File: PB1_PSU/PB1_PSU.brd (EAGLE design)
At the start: 100 x 80 mm, 0 parts

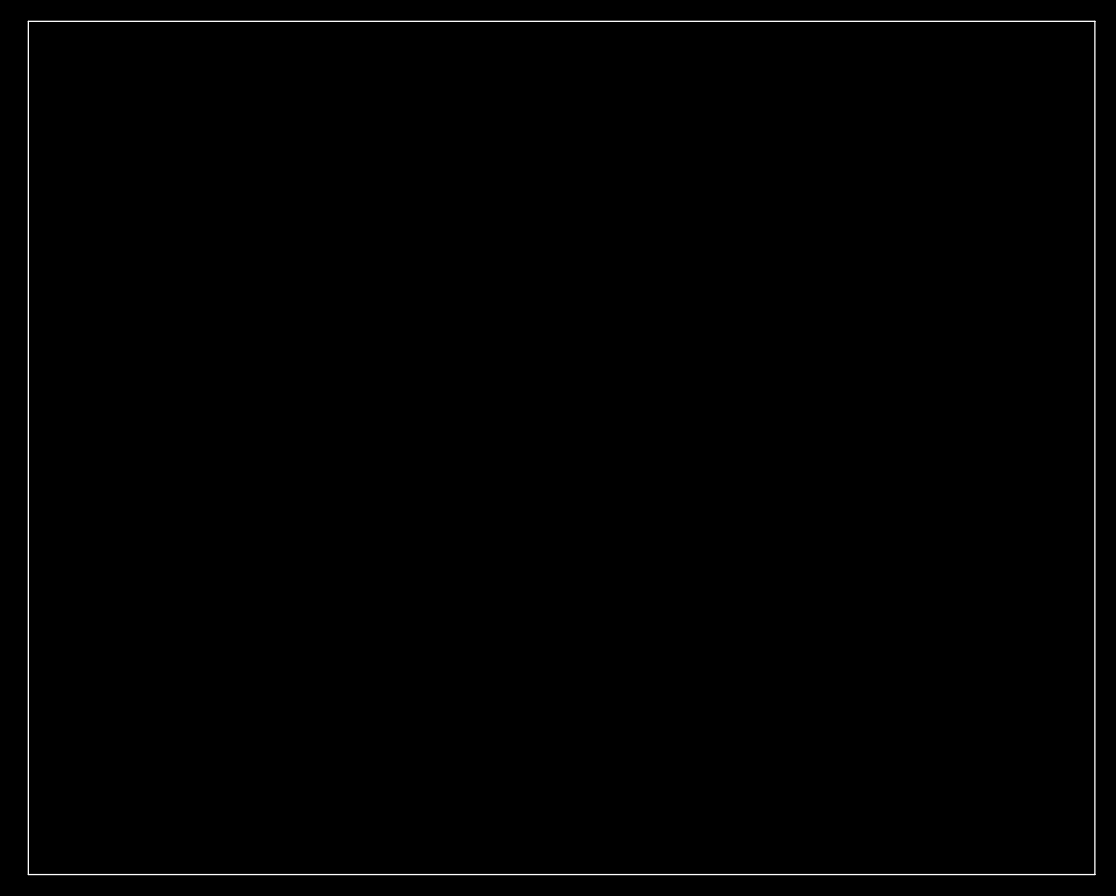
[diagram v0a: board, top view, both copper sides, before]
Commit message: * started on the PB1 powersupply
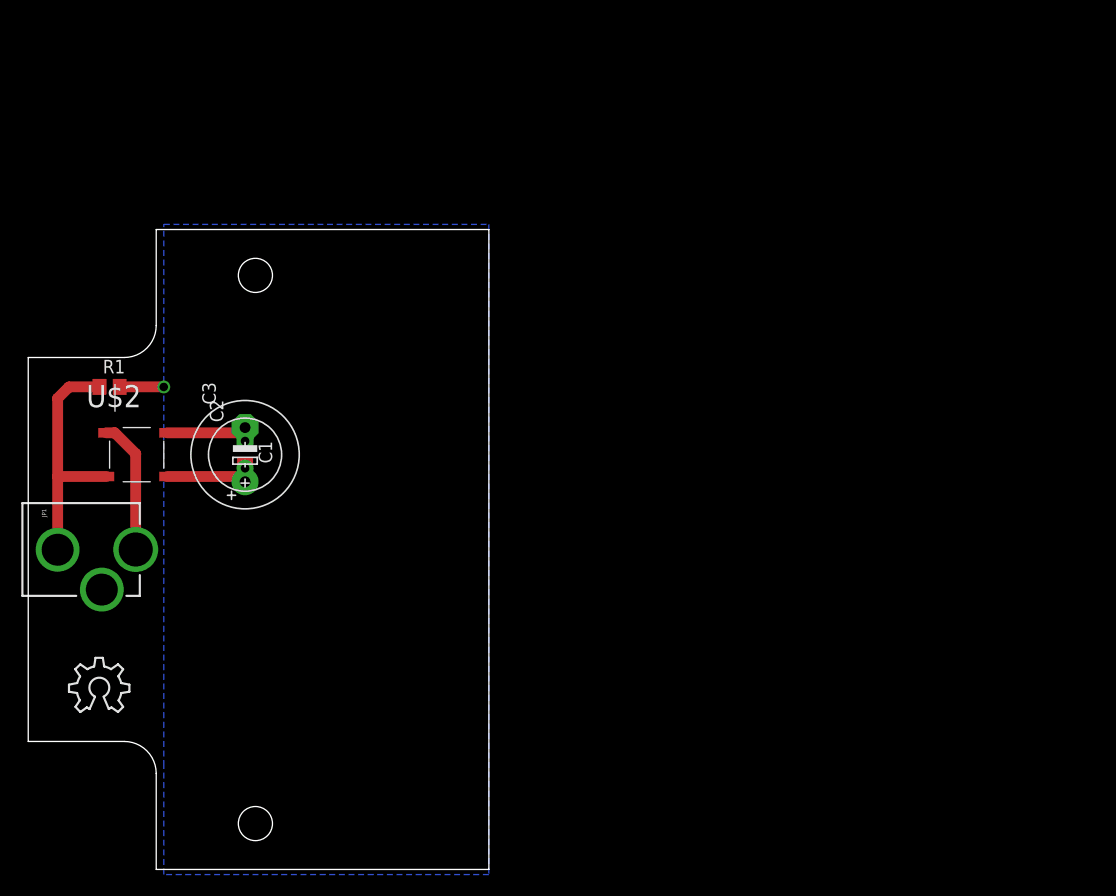
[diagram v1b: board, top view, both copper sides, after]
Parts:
- added C1: (no value), SquantorRCL:C0805
- added C2: (no value), SquantorRCL:E2,5-7
- added C3: (no value), SquantorRCL:E5-10,5
- added JP1: POWER_JACKPTH_LOCK, SquantorConnectors:POWER_JACK_PTH_LOCK
- added LOGO1: OSHW_LOGO_8MILX0200-NT, ohw-logo:OSHW_8X200_NOTEXT
- added R1: (no value), SquantorRCL:R0805
- added U$1: FUTURLEC_PB1PB1_HALF, SquantorPCBOutline:FUTURLEC_PB1_HALF
- added U$2: BRIDGE_RECTIFIERABS, SquantorDiodes:ABS
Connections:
- new net AC_EDGE: JP1.GND, R1.1, U$2.AC@2
- new net AC_PIN: JP1.PWR, U$2.AC@1
- new net AC_SW: JP1.GNDBREAK
- new net GND: C1.1, C2.-, C3.-, R1.2, U$2.-
- new net VRECT: C1.2, C2.+, C3.+, U$2.+
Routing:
- net AC_EDGE: track 0.00 -> 23.1 mm
- net AC_PIN: track 0.00 -> 12.6 mm
- net GND: track 0.00 -> 12.2 mm, vias 0 -> 1
- net VRECT: track 0.00 -> 8.89 mm
- added copper zone on layer 16, net GND
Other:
- board size 100 x 80 mm -> 43.2 x 60 mm
